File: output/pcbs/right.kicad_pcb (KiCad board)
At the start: 2 copper layers, 139.8 x 121.8 mm, 63 parts

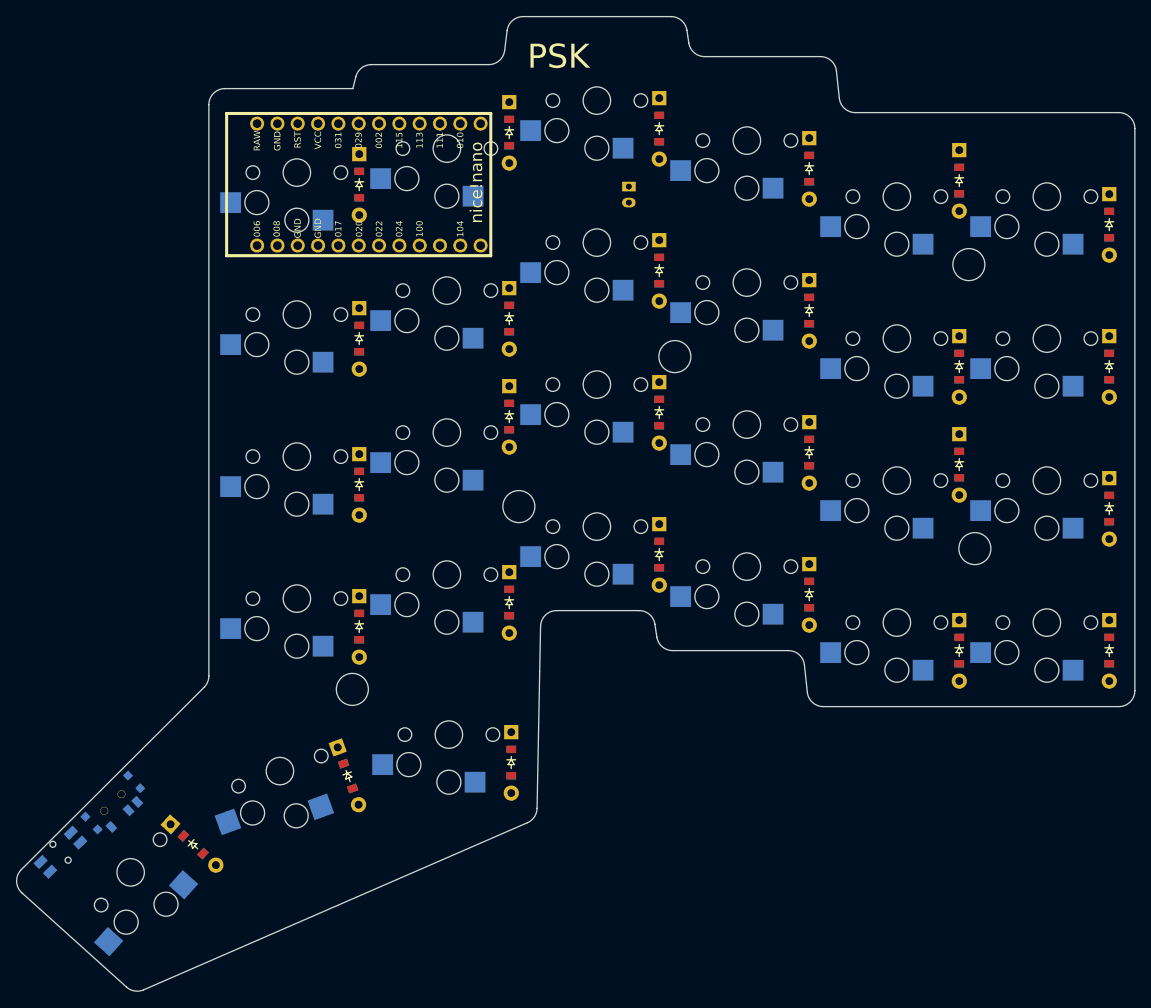
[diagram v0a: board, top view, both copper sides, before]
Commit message: wip routing right board
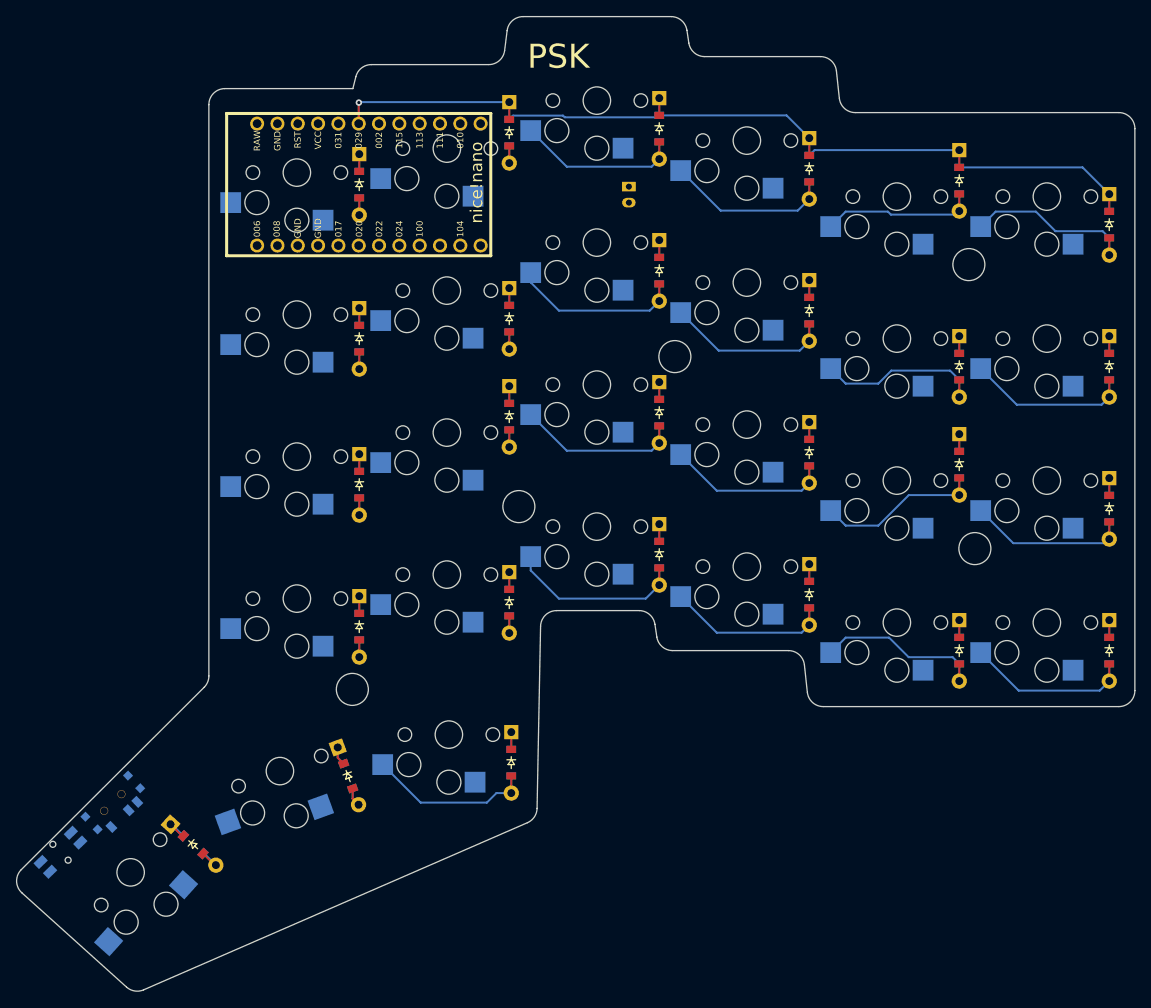
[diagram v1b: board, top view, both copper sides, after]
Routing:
- net P029: track 0.00 -> 125.6 mm, vias 0 -> 1
- net P115: track 0.00 -> 25.9 mm
- net P113: track 0.00 -> 25.9 mm
- net P002: track 0.00 -> 25.9 mm
- net mirror_fourth_mod: track 0.00 -> 24.3 mm
- net mirror_fourth_home: track 0.00 -> 23.6 mm
- net mirror_third_top: track 0.00 -> 23.1 mm
- net mirror_third_home: track 0.00 -> 22.9 mm
- net mirror_near_thumb: track 0.00 -> 22.9 mm
- net mirror_first_mod: track 0.00 -> 22.9 mm
- net mirror_second_bottom: track 0.00 -> 22.8 mm
- net mirror_fourth_top: track 0.00 -> 22.7 mm
- net mirror_first_home: track 0.00 -> 22.7 mm
- net mirror_third_mod: track 0.00 -> 22.7 mm
- net mirror_third_bottom: track 0.00 -> 22.7 mm
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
